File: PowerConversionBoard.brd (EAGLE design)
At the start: 152.4 x 101.6 mm, 48 parts, among them U1 LM2678, U2 LM2678

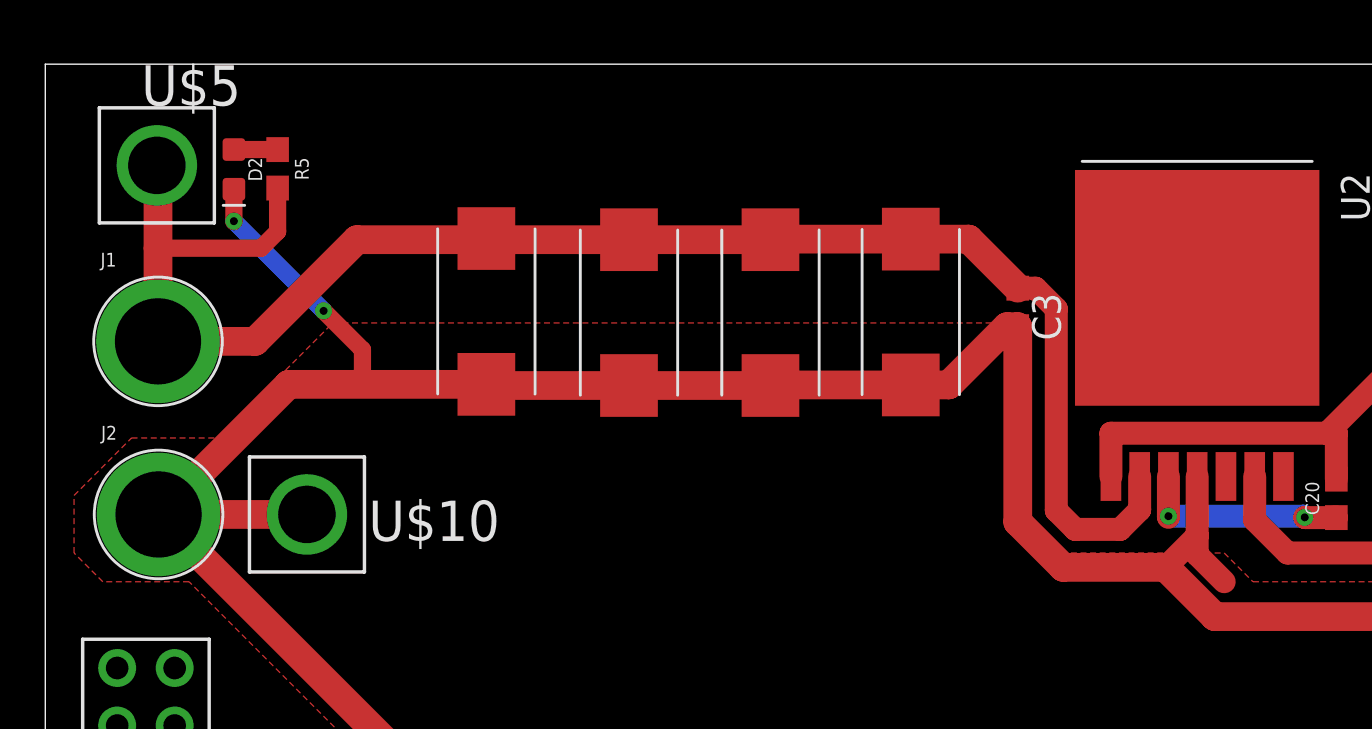
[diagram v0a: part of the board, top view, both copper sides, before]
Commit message: plane ez
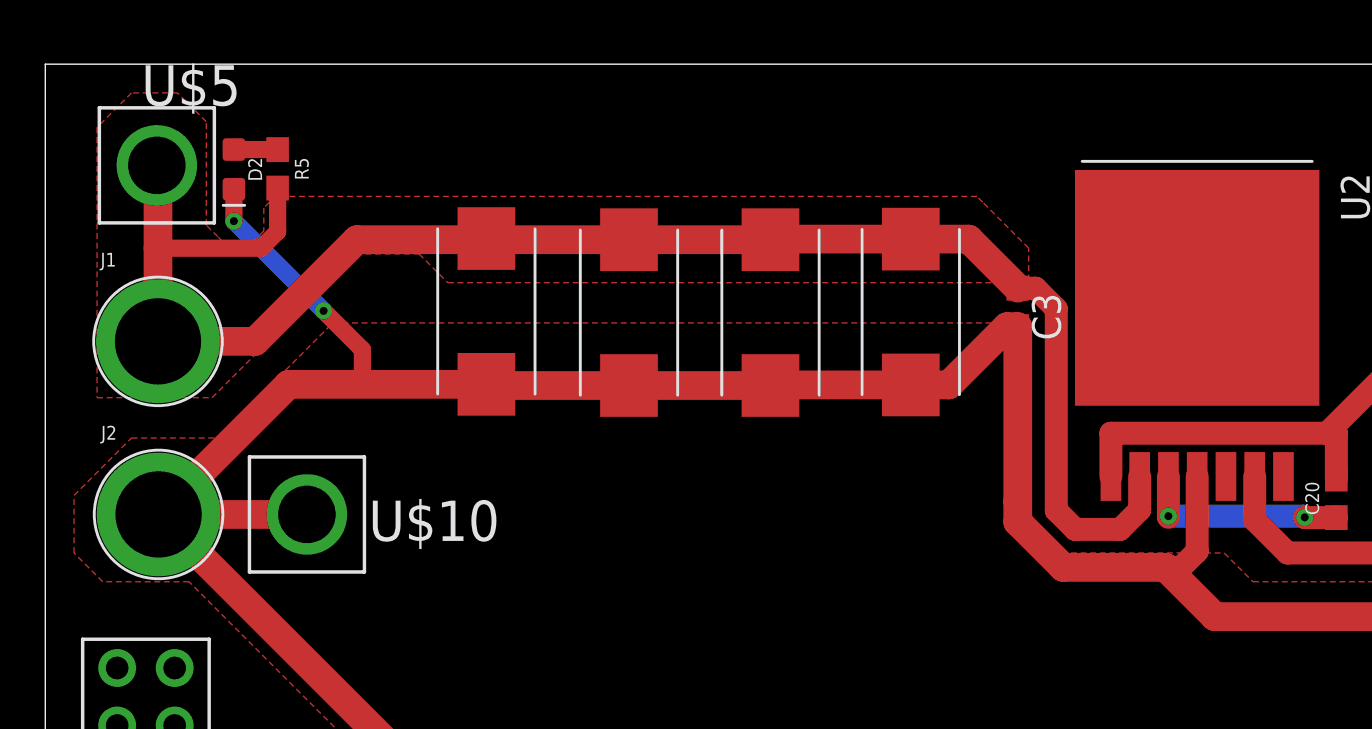
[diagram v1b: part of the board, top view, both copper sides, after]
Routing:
- net GND: track 411.0 -> 408.9 mm
- added copper zone on layer 1, net +12V
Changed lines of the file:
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@@
 <setting verticaltext="up"/>
 </settings>
-<grid distance="50" unitdist="mil" unit="mil" style="lines" multiple="1" display="yes" altdistance="5" altunitdist="mil" altunit="inch"/>
+<grid distance="10" unitdist="mil" unit="mil" style="lines" multiple="1" display="yes" altdistance="5" altunitdist="mil" altunit="inch"/>
 <layers>
 <layer number="1" name="Top" color="4" fill="1" visible="yes" active="yes"/>
@@
 <contactref element="U$9" pad="8"/>
 <contactref element="U$9" pad="10"/>
-<wire x1="5.715" y1="74.93" x2="4.9784" y2="89.3572" width="0" layer="19" extent="1-1"/>
+<polygon width="0.254" layer="1">
+<vertex x="2.286" y="86.868"/>
+<vertex x="7.366" y="86.868"/>
+<vertex x="13.716" y="93.218"/>
+<vertex x="16.51" y="93.218"/>
+<vertex x="17.78" y="91.948"/>
+<vertex x="41.91" y="91.948"/>
+<vertex x="42.672" y="91.186"/>
+<vertex x="43.434" y="91.186"/>
+<vertex x="43.434" y="93.472"/>
+<vertex x="41.402" y="95.504"/>
+<vertex x="41.148" y="95.758"/>
+<vertex x="10.16" y="95.758"/>
+<vertex x="9.906" y="95.504"/>
+<vertex x="9.652" y="95.25"/>
+<vertex x="9.652" y="94.234"/>
+<vertex x="8.89" y="93.472"/>
+<vertex x="8.128" y="93.472"/>
+<vertex x="7.62" y="93.98"/>
+<vertex x="7.112" y="94.488"/>
+<vertex x="7.112" y="99.06"/>
+<vertex x="5.842" y="100.33"/>
+<vertex x="3.81" y="100.33"/>
+<vertex x="2.286" y="98.806"/>
+</polygon>
 <wire x1="5.715" y1="72.39" x2="5.715" y2="74.93" width="0" layer="19" extent="1-1"/>
 <wire x1="3.175" y1="74.93" x2="5.715" y2="74.93" width="0" layer="19" extent="1-1"/>
@@
 <wire x1="3.175" y1="64.77" x2="5.715" y2="64.77" width="0" layer="19" extent="1-1"/>
 <wire x1="3.175" y1="62.23" x2="5.715" y2="62.23" width="0" layer="19" extent="1-1"/>
+<wire x1="4.9784" y1="89.3572" x2="5.715" y2="74.93" width="0" layer="19" extent="1-1"/>
 </signal>
 <signal name="GND">
@@
 <wire x1="19.3294625" y1="67.3861375" x2="19.3294" y2="60.6748" width="1.27" layer="1"/>
 <wire x1="43.0784" y1="89.8788" x2="42.9514" y2="90.0058" width="1.016" layer="1"/>
-<wire x1="50.8762" y1="83.3882" x2="50.8762" y2="80.772" width="1.016" layer="1"/>
-<wire x1="42.9514" y1="90.0058" x2="42.9514" y2="81.3816" width="1.27" layer="1"/>
-<wire x1="44.958" y1="79.375" x2="42.9514" y2="81.3816" width="1.27" layer="1"/>
+<wire x1="42.9514" y1="81.3816" x2="44.958" y2="79.375" width="1.27" layer="1"/>
 <wire x1="49.4792" y1="79.375" x2="44.958" y2="79.375" width="1.27" layer="1"/>
-<wire x1="50.8762" y1="80.772" x2="49.4792" y2="79.375" width="1.016" layer="1"/>
 <wire x1="10.75" y1="87.458" x2="5.0038" y2="81.7118" width="1.27" layer="1"/>
 <wire x1="19.4818" y1="87.458" x2="10.75" y2="87.458" width="1.27" layer="1"/>
@@
 <vertex x="1.27" y="80.01"/>
 </polygon>
-<wire x1="50.8762" y1="80.772" x2="50.8762" y2="79.9338" width="1.016" layer="1"/>
-<wire x1="50.8762" y1="79.9338" x2="52.07" y2="78.74" width="1.016" layer="1"/>
+<wire x1="42.9514" y1="90.0058" x2="42.9514" y2="82.296" width="1.27" layer="1"/>
+<wire x1="42.9514" y1="82.296" x2="42.9514" y2="81.3816" width="1.27" layer="1"/>
+<wire x1="50.8762" y1="83.3882" x2="50.8762" y2="80.0862" width="1.016" layer="1"/>
+<wire x1="50.8762" y1="80.0862" x2="50.8" y2="80.01" width="1.016" layer="1"/>
+<wire x1="50.8" y1="80.01" x2="50.165" y2="79.375" width="1.016" layer="1"/>
+<wire x1="50.165" y1="79.375" x2="49.4792" y2="79.375" width="1.016" layer="1"/>
 <wire x1="122.6312" y1="82.6196" x2="122.6312" y2="93.2196" width="0" layer="19" extent="1-1"/>
-<wire x1="50.8762" y1="91.7194" x2="43.0784" y2="89.8788" width="0" layer="19" extent="1-1"/>
+<wire x1="14.0081" y1="87.5411" x2="19.4818" y2="87.458" width="0" layer="19" extent="1-1"/>
+<wire x1="42.9514" y1="82.296" x2="50.8762" y2="91.7194" width="0" layer="19" extent="1-1"/>
+<wire x1="51.054" y1="59.5122" x2="51.054" y2="51.181" width="0" layer="19" extent="1-1"/>
 <wire x1="5.715" y1="59.69" x2="19.3294" y2="60.6748" width="0" layer="19" extent="1-1"/>
 <wire x1="5.715" y1="57.15" x2="5.715" y2="59.69" width="0" layer="19" extent="1-1"/>
